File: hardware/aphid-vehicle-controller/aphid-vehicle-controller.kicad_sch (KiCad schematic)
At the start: 0 parts

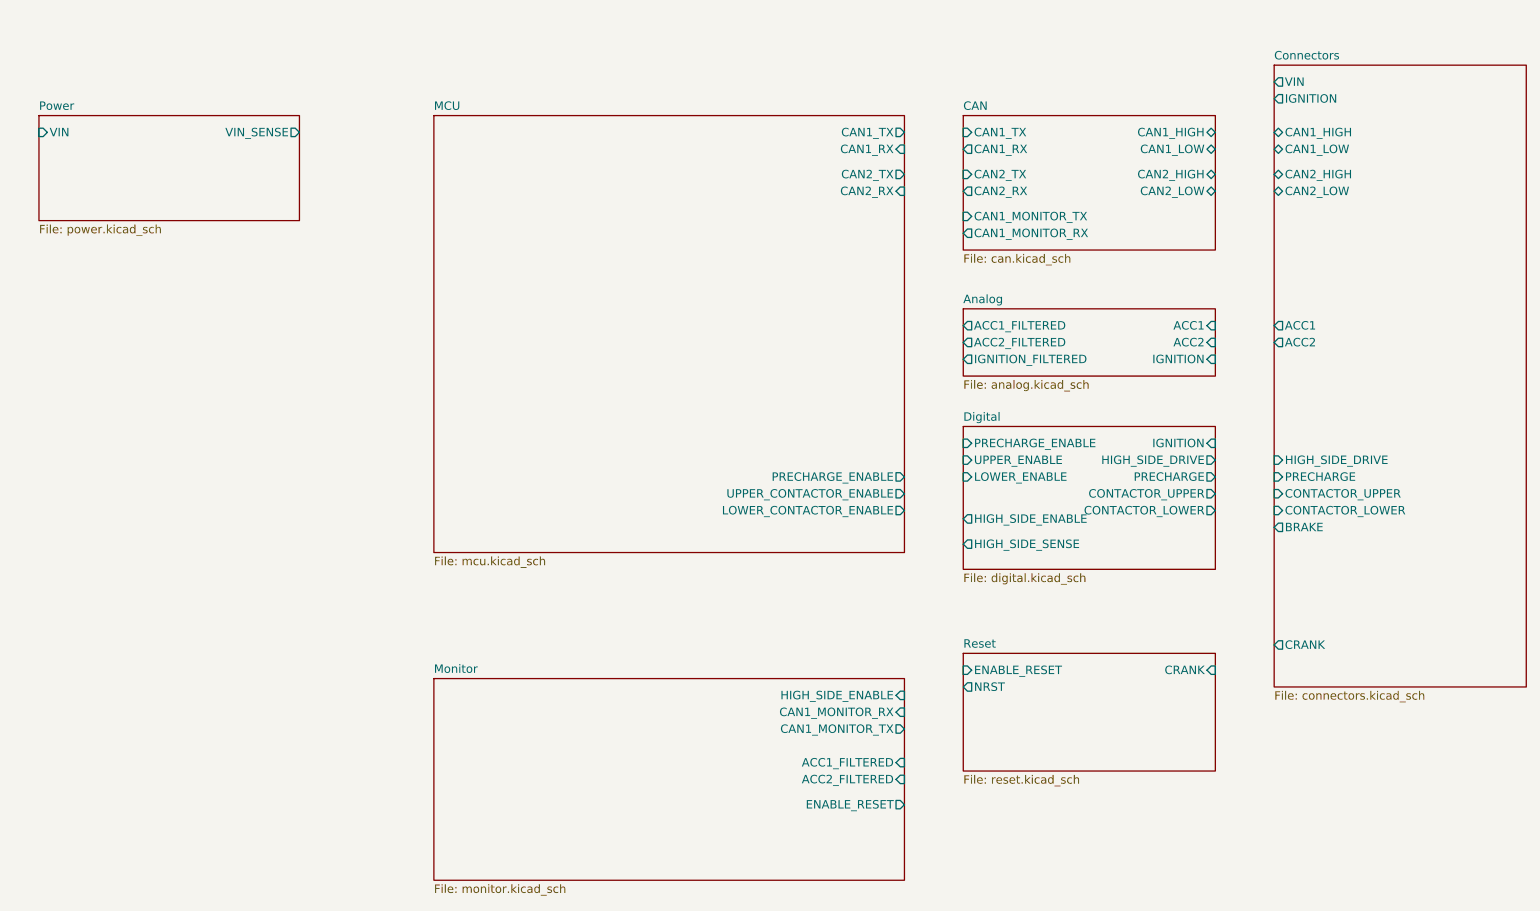
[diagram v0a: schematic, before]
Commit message: worked on VCM
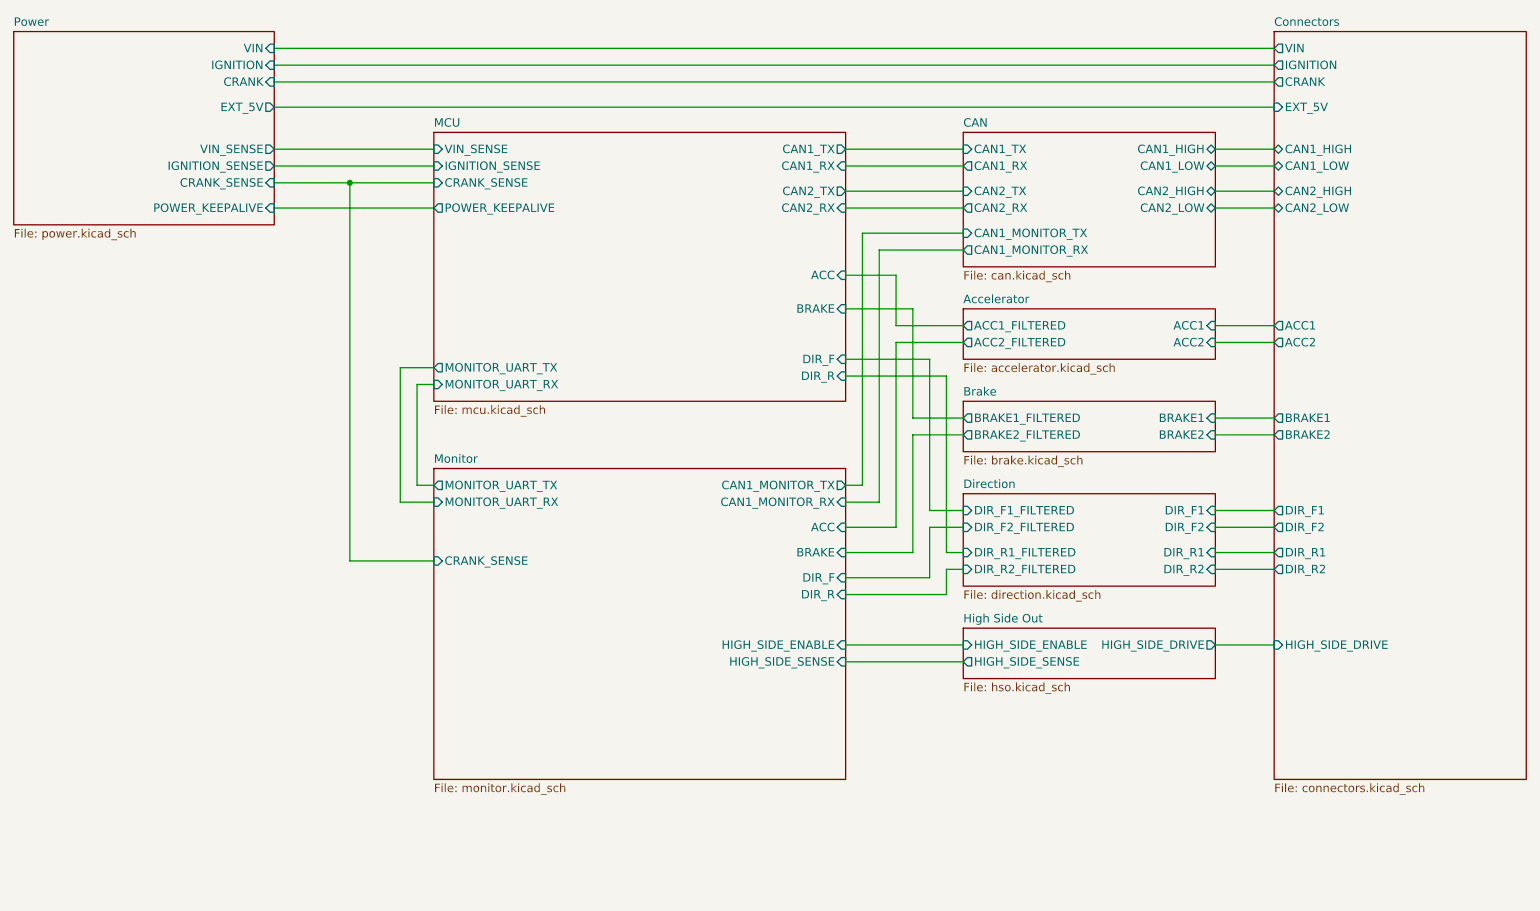
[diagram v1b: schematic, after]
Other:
- sheet Analog renamed Accelerator
- sheet Digital renamed High Side Out
- removed sheet Reset
- added sheet Brake (brake.kicad_sch)
- added sheet Direction (direction.kicad_sch)
- sheet Accelerator: file analog.kicad_sch -> accelerator.kicad_sch
- sheet Accelerator ports: added none; removed IGNITION, IGNITION_FILTERED
- sheet Connectors ports: added BRAKE1, BRAKE2, DIR_F1, DIR_F2, DIR_R1, DIR_R2, EXT_5V; removed BRAKE, CONTACTOR_LOWER, CONTACTOR_UPPER, PRECHARGE
- sheet High Side Out: file digital.kicad_sch -> hso.kicad_sch
- sheet High Side Out ports: added none; removed CONTACTOR_LOWER, CONTACTOR_UPPER, IGNITION, LOWER_ENABLE, PRECHARGE, PRECHARGE_ENABLE, UPPER_ENABLE
- sheet MCU ports: added ACC, BRAKE, CRANK_SENSE, DIR_F, DIR_R, IGNITION_SENSE, MONITOR_UART_RX, MONITOR_UART_TX, POWER_KEEPALIVE, VIN_SENSE; removed LOWER_CONTACTOR_ENABLE, PRECHARGE_ENABLE, UPPER_CONTACTOR_ENABLE
- sheet Monitor ports: added ACC, BRAKE, CRANK_SENSE, DIR_F, DIR_R, HIGH_SIDE_SENSE, MONITOR_UART_RX, MONITOR_UART_TX; removed ACC1_FILTERED, ACC2_FILTERED, ENABLE_RESET
- sheet Power ports: added CRANK, CRANK_SENSE, EXT_5V, IGNITION, IGNITION_SENSE, POWER_KEEPALIVE; removed none
